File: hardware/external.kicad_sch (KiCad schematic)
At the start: 10 parts, among them J4 Conn_02x04_Odd_Even, J8 Conn_01x04_Pin, J9 Conn_01x04_Pin

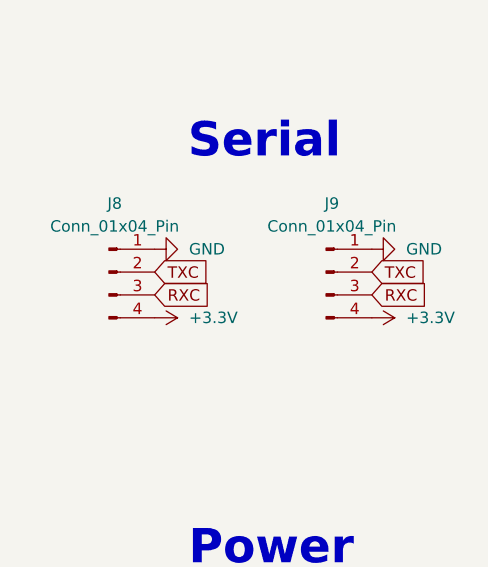
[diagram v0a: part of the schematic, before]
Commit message: Minor Improvemnts
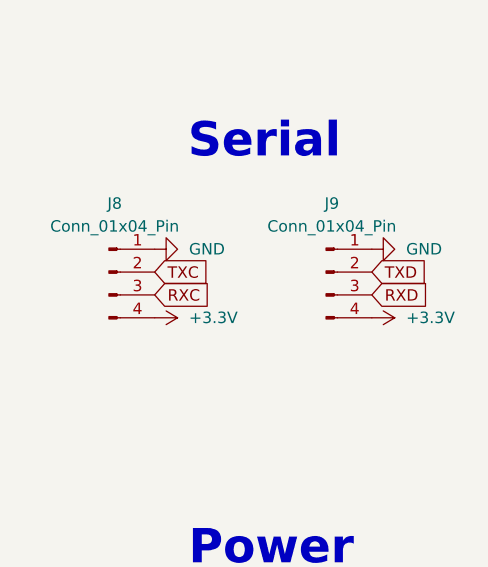
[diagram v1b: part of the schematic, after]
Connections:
- net RXC: no longer J9.3 (Pin_3)
- net TXC: no longer J9.2 (Pin_2)
- new net RXD: J9.3 (Pin_3)
- new net TXD: J9.2 (Pin_2)
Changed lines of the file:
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@@
 		)
 	)
-	(global_label "TXC"
+	(global_label "TXD"
 		(shape input)
 		(at 236.22 93.98 0)
@@
 		)
 	)
-	(global_label "RXC"
+	(global_label "RXD"
 		(shape input)
 		(at 236.22 96.52 0)
